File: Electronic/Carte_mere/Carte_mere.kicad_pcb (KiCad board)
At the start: 2 copper layers, 85 x 65 mm, 60 parts, among them J1 USB_C_Receptacle_USB2.0_14P, J10 Conn_01x07, J11 Conn_01x08, J2 Conn_01x04, J3 Conn_01x02, J4 Conn_01x02, J5 Conn_01x07, J6 Conn_01x07, J7 xt60pm, J8 Conn_01x11, J9 Conn_01x07, SW1 push button, SW2 push button RST, U1 TPS5431DDA, U2 ESP32-S3-WROOM-2, U3 TPS5431DDA

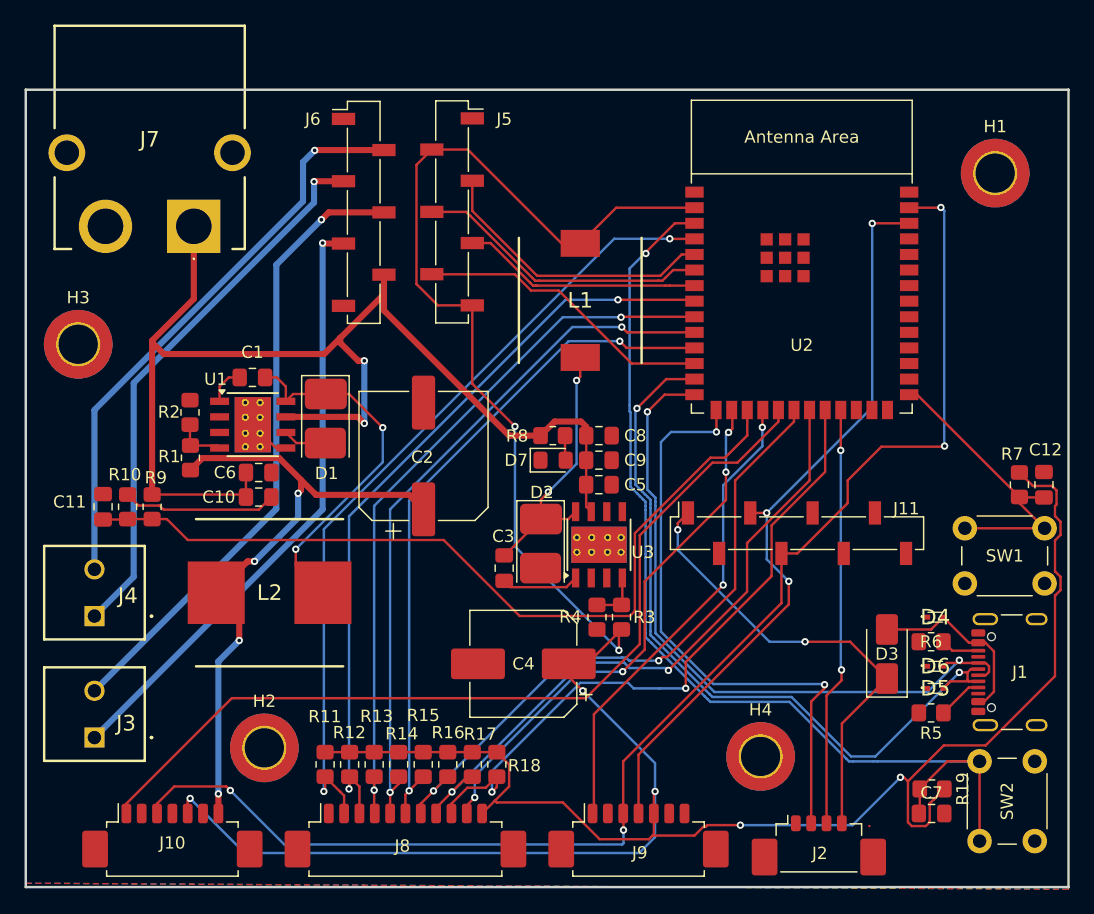
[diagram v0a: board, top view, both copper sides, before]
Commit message: Add files via upload
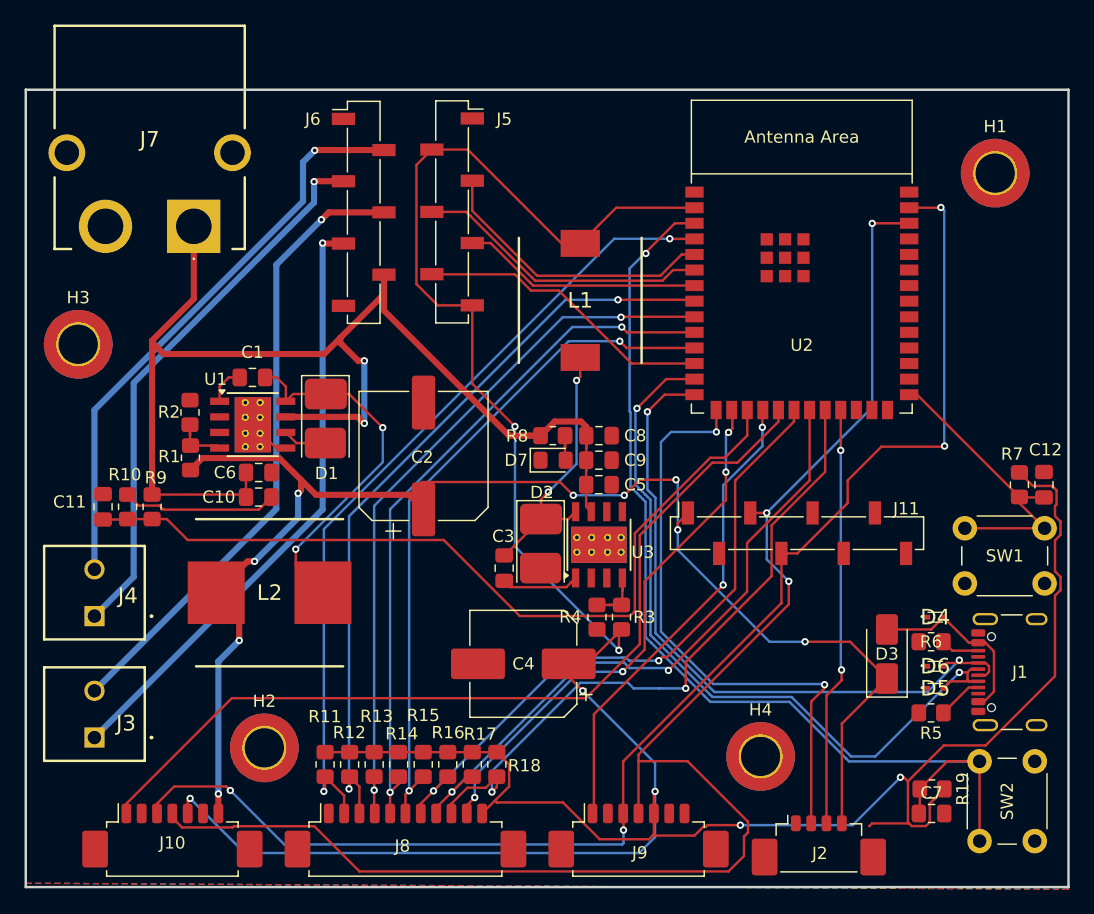
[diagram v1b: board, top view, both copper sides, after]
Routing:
- net SCL: track 61.8 -> 125.1 mm
- net +5V: track 91.6 -> 118.9 mm, vias 6 -> 9
- net +3.3V: track 248.3 -> 252.5 mm
- net LIPO11V1: track 100.7 -> 104.0 mm
- net Net-(U3-VSENSE): track 4.23 -> 6.29 mm
- net Net-(D7-A): track 2.02 -> 3.03 mm
- net Net-(U1-VSENSE): track 4.18 -> 5.01 mm
- net Net-(U3-BOOT): track 6.35 -> 6.88 mm
